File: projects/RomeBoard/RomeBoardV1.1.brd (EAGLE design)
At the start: 110 x 135 mm, 27 parts, among them J1 HEADER-5, J2 RASPBERRY-PI-HEADER, M1 2N7000, M2 2N7000, M3 2N7000, U1 LM1084IT-ADJ

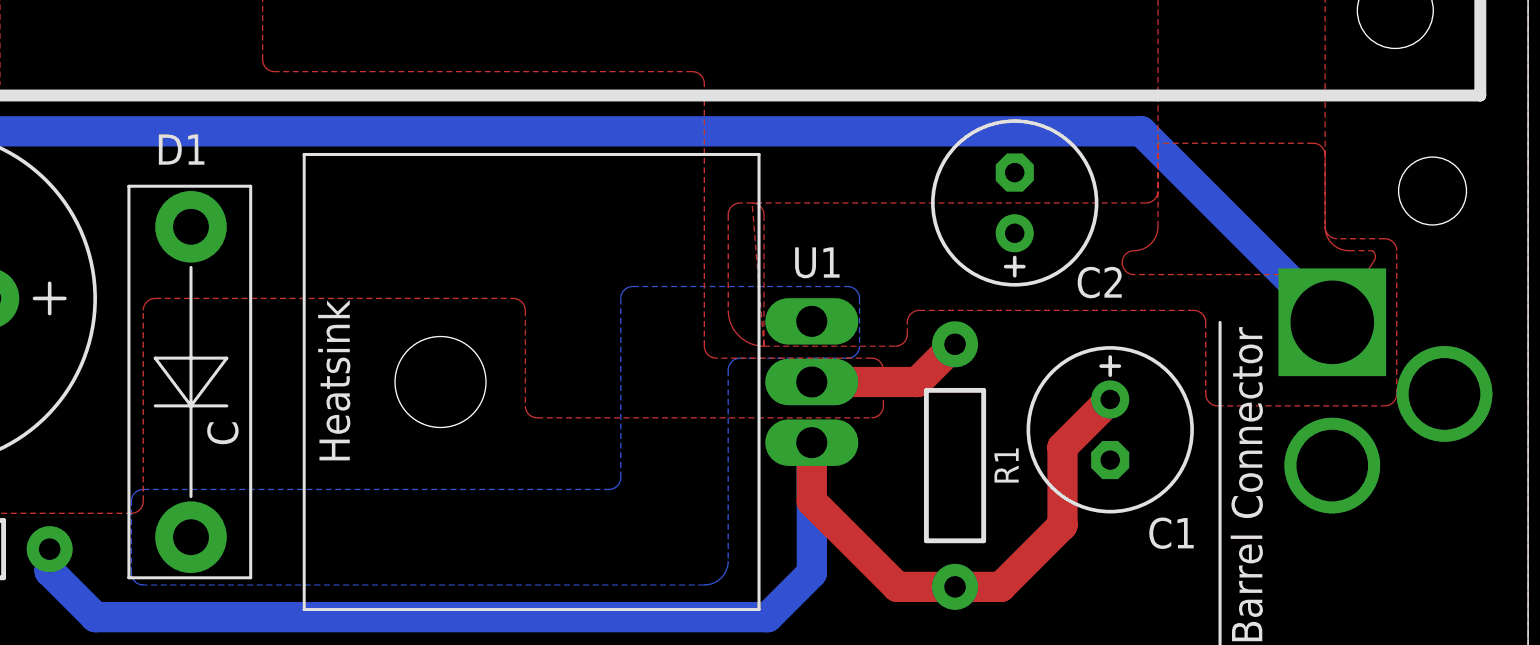
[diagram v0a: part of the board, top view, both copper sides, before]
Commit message: fixing air wire + updating library
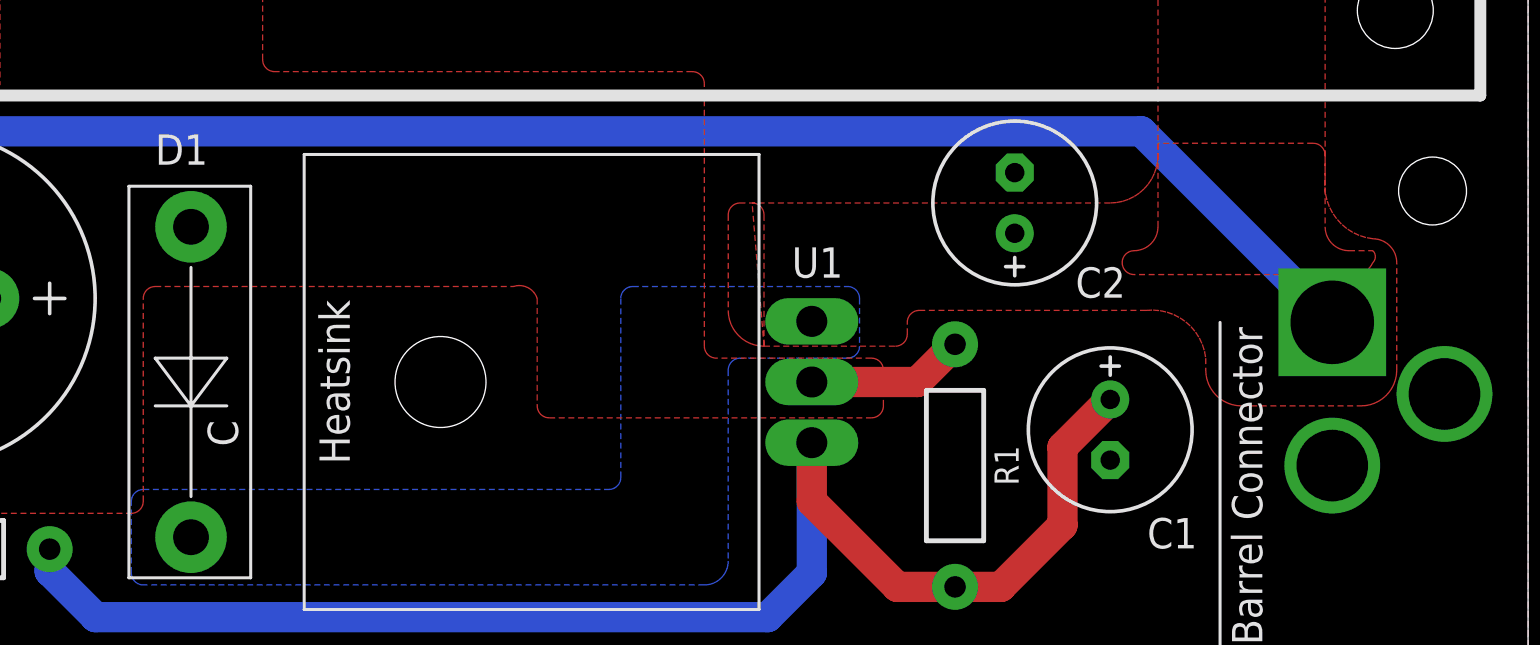
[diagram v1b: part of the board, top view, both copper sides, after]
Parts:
- M1, M2, M3: value 2N7000 -> ZVN4424A
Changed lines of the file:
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@@
 <element name="R6" library="passives" package="AXIAL-0.4" value="147R" x="5" y="46" rot="R270"/>
 <element name="R7" library="passives" package="AXIAL-0.4" value="147R" x="32" y="34" rot="R270"/>
-<element name="M1" library="BrownSpaceEngineering" package="TO-923-MOS" value="2N7000" x="26" y="63" rot="R270"/>
-<element name="M2" library="BrownSpaceEngineering" package="TO-923-MOS" value="2N7000" x="12" y="51" rot="R270"/>
-<element name="M3" library="BrownSpaceEngineering" package="TO-923-MOS" value="2N7000" x="26" y="39" rot="R270"/>
+<element name="M1" library="BrownSpaceEngineering" package="TO-923-MOS" value="ZVN4424A" x="26" y="63" rot="R270"/>
+<element name="M2" library="BrownSpaceEngineering" package="TO-923-MOS" value="ZVN4424A" x="12" y="51" rot="R270"/>
+<element name="M3" library="BrownSpaceEngineering" package="TO-923-MOS" value="ZVN4424A" x="26" y="39" rot="R270"/>
 <element name="R8" library="passives" package="AXIAL-0.4" value="10K" x="105" y="78" rot="R270"/>
 <element name="U1" library="BrownSpaceEngineering" package="TO-220-507302B00000G" value="LM1084IT-ADJ" x="80" y="11.5" smashed="yes" rot="R90">
@@
 <vertex x="51.5" y="6" curve="90"/>
 <vertex x="52" y="6.5"/>
-<vertex x="52" y="14.5" curve="-90"/>
-<vertex x="52.5" y="15"/>
-<vertex x="67.5" y="15" curve="-90"/>
-<vertex x="68" y="14.5"/>
-<vertex x="68" y="10.5" curve="90"/>
-<vertex x="68.5" y="10"/>
+<vertex x="52" y="15" curve="-90"/>
+<vertex x="52.5" y="15.5"/>
+<vertex x="67.5" y="15.5" curve="-90"/>
+<vertex x="68.5" y="15"/>
+<vertex x="68.5" y="10.5" curve="90"/>
+<vertex x="69" y="10"/>
 <vertex x="82.5" y="10" curve="90"/>
 <vertex x="83" y="10.5"/>
@@
 <polygon width="0.254" layer="1" isolate="0.3048" thermals="no">
 <vertex x="94.5" y="21.5"/>
-<vertex x="94.5" y="19.5" curve="-90"/>
-<vertex x="94" y="19"/>
+<vertex x="94.5" y="21" curve="-90"/>
+<vertex x="92.5" y="19"/>
 <vertex x="77" y="19" curve="90"/>
 <vertex x="76.5" y="18.5"/>
@@
 <vertex x="84" y="14" curve="-90"/>
 <vertex x="84.5" y="14.5"/>
-<vertex x="96" y="14.5" curve="-90"/>
-<vertex x="96.5" y="14"/>
-<vertex x="96.5" y="11" curve="90"/>
-<vertex x="97" y="10.5"/>
-<vertex x="104" y="10.5" curve="90"/>
-<vertex x="104.5" y="11"/>
-<vertex x="104.5" y="17" curve="90"/>
-<vertex x="104" y="17.5"/>
-<vertex x="102" y="17.5" curve="-90"/>
-<vertex x="101.5" y="18"/>
+<vertex x="94" y="14.5" curve="-90"/>
+<vertex x="96.5" y="12.5"/>
+<vertex x="96.5" y="12" curve="90"/>
+<vertex x="98" y="10.5"/>
+<vertex x="103" y="10.5" curve="90"/>
+<vertex x="104.5" y="12"/>
+<vertex x="104.5" y="16.5" curve="90"/>
+<vertex x="103.5" y="17.5" curve="-90"/>
+<vertex x="101.5" y="20"/>
 <vertex x="101.5" y="21" curve="90"/>
 <vertex x="101" y="21.5"/>
